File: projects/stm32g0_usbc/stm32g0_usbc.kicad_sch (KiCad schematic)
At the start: 27 parts, among them J1 USB_C_Receptacle_USB2.0, J3 Conn_ARM_JTAG_SWD_10, U1 STM32G0B1CBT, U2 MCP1754S-3302xMB, U3 8MHz 20pF ±10ppm, Y2 NX3225GD 8 MHz

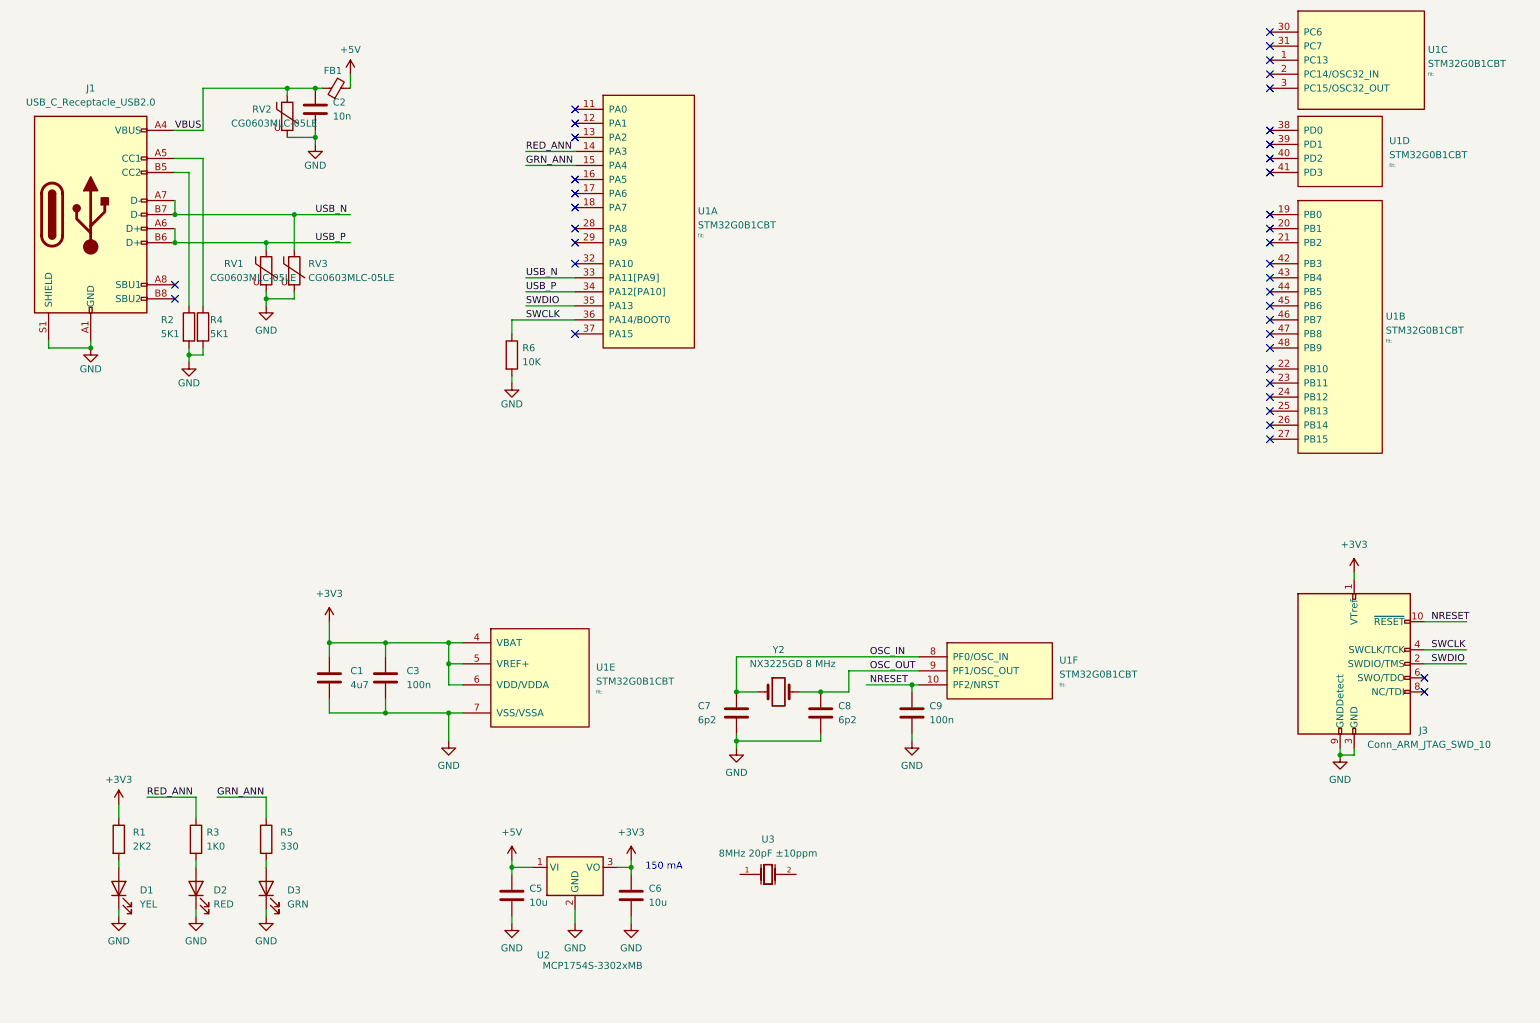
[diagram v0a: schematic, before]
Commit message: .
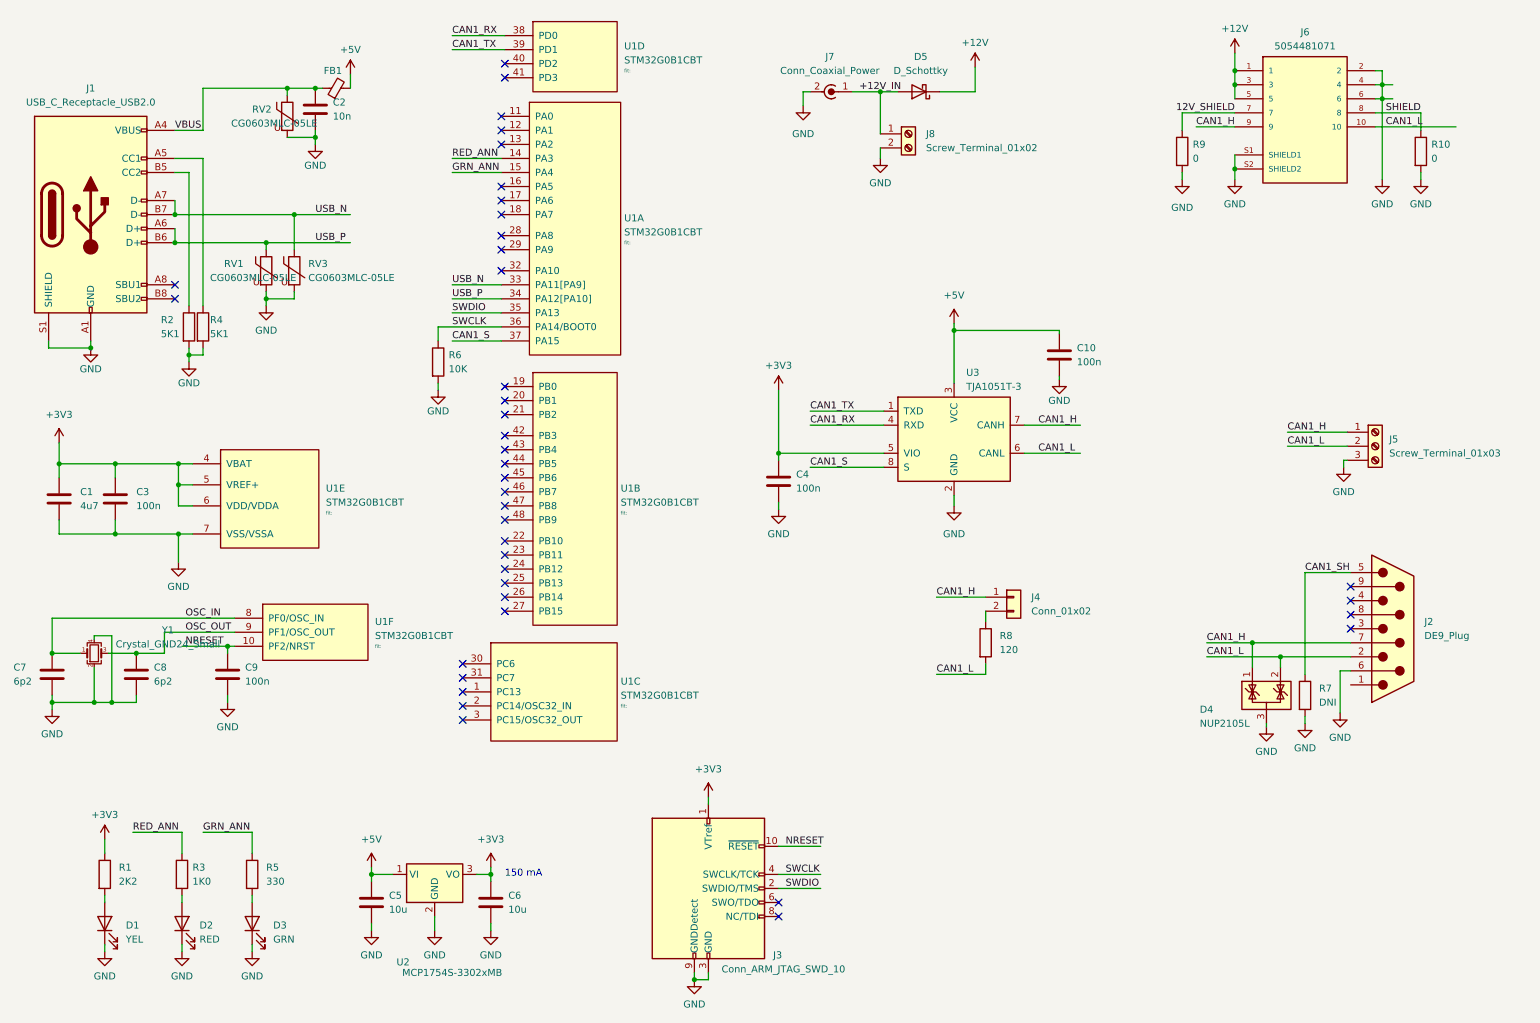
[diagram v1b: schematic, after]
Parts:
- removed U3: 8MHz 20pF ±10ppm, JLCPCB:OSC-SMD_L5.0-W3.2, symbol JLCPCB Chips, Crystals:8MHz 20pF ±10ppm
- removed Y2: NX3225GD 8 MHz, Crystal:Crystal_SMD_3215-2Pin_3.2x1.5mm, symbol Device:Crystal
- added C10, C4: 100n, Capacitor_SMD:C_0603_1608Metric, symbol Device:C
- added D4: NUP2105L, Package_TO_SOT_SMD:SOT-23, symbol Power_Protection:NUP2105L
- added D5: D_Schottky, Diode_SMD:D_SMA, symbol Device:D_Schottky
- added J2: DE9_Plug, Connector_Dsub:DSUB-9_Male_Horizontal_P2.77x2.84mm_EdgePinOffset4.94mm_Housed_MountingHolesOffset7.48mm, symbol Connector:DE9_Plug
- added J4: Conn_01x02, Connector_PinHeader_2.54mm:PinHeader_1x02_P2.54mm_Vertical, symbol Connector_Generic:Conn_01x02
- added J5: Screw_Terminal_01x03, TerminalBlock_Phoenix:TerminalBlock_Phoenix_MKDS-1,5-3_1x03_P5.00mm_Horizontal, symbol Connector:Screw_Terminal_01x03
- added J6: 5054481071, molex_microlock_plus:MOLEX_5054481071, symbol molex_microlock_plus:5054481071
- added J7: Conn_Coaxial_Power, Connector_BarrelJack:BarrelJack_CUI_PJ-063AH_Horizontal, symbol Connector:Conn_Coaxial_Power
- added J8: Screw_Terminal_01x02, TerminalBlock_Phoenix:TerminalBlock_Phoenix_MKDS-1,5-2-5.08_1x02_P5.08mm_Horizontal, symbol Connector:Screw_Terminal_01x02
- added R10, R9: 0, Resistor_SMD:R_1206_3216Metric, symbol Device:R
- added R7: DNI, Resistor_SMD:R_1206_3216Metric, symbol Device:R
- added R8: 120, Resistor_SMD:R_1206_3216Metric, symbol Device:R
- added U3: TJA1051T-3, Package_SO:SOIC-8_3.9x4.9mm_P1.27mm, symbol Interface_CAN_LIN:TJA1051T-3
- added Y1: Crystal_GND24_Small, Crystal:Crystal_SMD_3225-4Pin_3.2x2.5mm, symbol Device:Crystal_GND24_Small
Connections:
- net +3V3: now also C4.1, U3.5 (VIO)
- net +5V: now also C10.1, U3.3 (VCC)
- net GND: now also C10.2, C4.2, D4.3 (A), J2.6, J5.3 (Pin_3), J6.2, J6.4, J6.6, J6.S1 (SHIELD1), J6.S2 (SHIELD2), J7.2 (Ext), J8.2 (Pin_2), R10.2, R7.2, R9.2, U3.2 (GND), Y1.2, Y1.4
- net OSC_IN: now also Y1.1
- net OSC_OUT: now also Y1.3
- net CAN1_S: now reaches U1.37 (PA15)
- net CAN1_S: now also U3.8 (S)
- net CAN1_RX: now reaches U1.38 (PD0)
- net CAN1_RX: now also U3.4 (RXD)
- net CAN1_TX: now reaches U1.39 (PD1)
- net CAN1_TX: now also U3.1 (TXD)
- new net: J4.2 (Pin_2), R8.1
- new net +12V: D5.1 (K), J6.1, J6.3, J6.5
- new net +12V_IN: D5.2 (A), J7.1 (In), J8.1 (Pin_1)
- new net 12V_SHIELD: J6.7, R9.1
- new net CAN1_H: D4.1 (K), J2.7, J4.1 (Pin_1), J5.1 (Pin_1), J6.9, U3.7 (CANH)
- new net CAN1_L: D4.2 (K), J2.2, J5.2 (Pin_2), J6.10, R8.2, U3.6 (CANL)
- new net CAN1_SH: J2.5, R7.1
- new net SHIELD: J6.8, R10.1
- no-connect marks 39 -> 40
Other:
- moved on the sheet: C1, C3, C5, C6, C7, C8, C9, D1, D2, D3, J3, R1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
